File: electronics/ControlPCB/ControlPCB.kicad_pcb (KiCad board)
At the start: 2 copper layers, 119.6 x 90.4 mm, 44 parts, among them CON1 12VINPUT, P1 Opto1, P2 Opto2, P3 Opto3, P4 Opto4, P5 Opto5, P6 Opto6, P7 Tool, U1 POLOLU_A4988, U2 POLOLU_A4988, U3 POLOLU_A4988, U4 POLOLU_A4988, U5 POLOLU_A4988, U6 POLOLU_A4988, U7 POLOLU_A4988

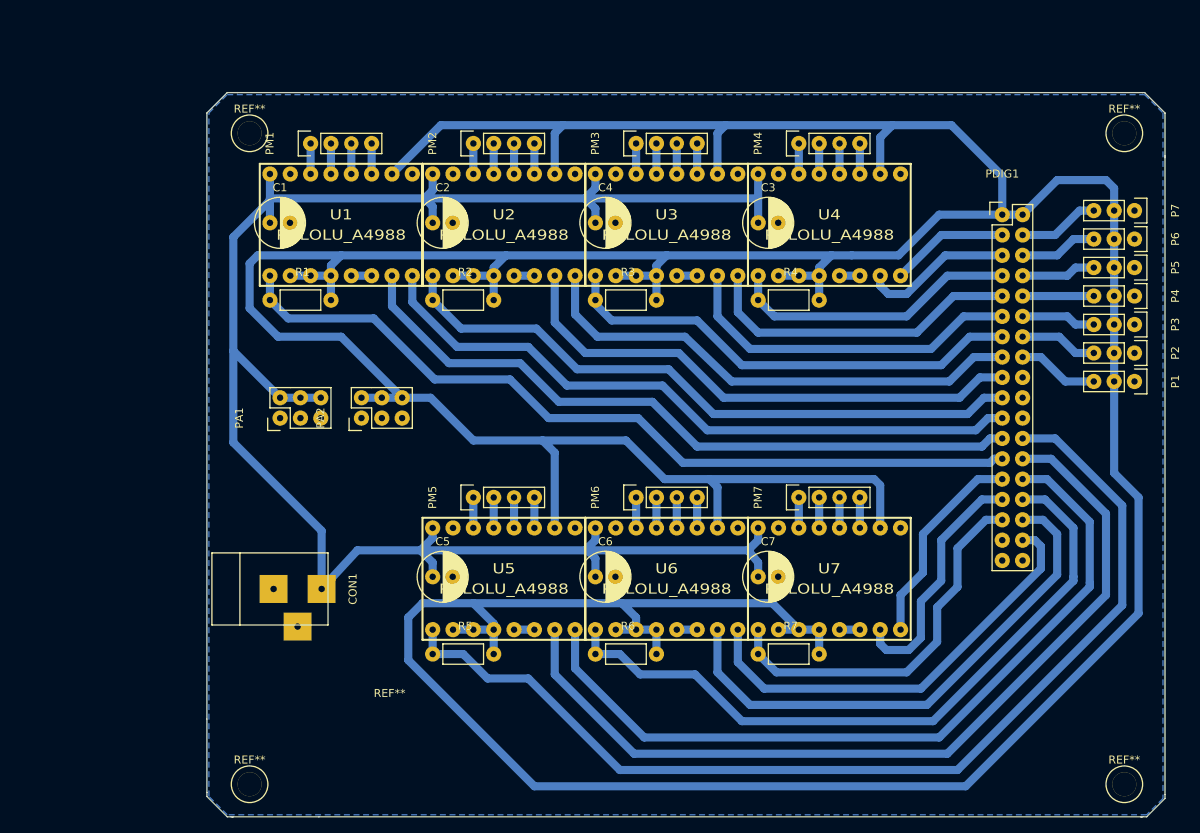
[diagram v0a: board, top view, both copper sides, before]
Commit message: PCB update
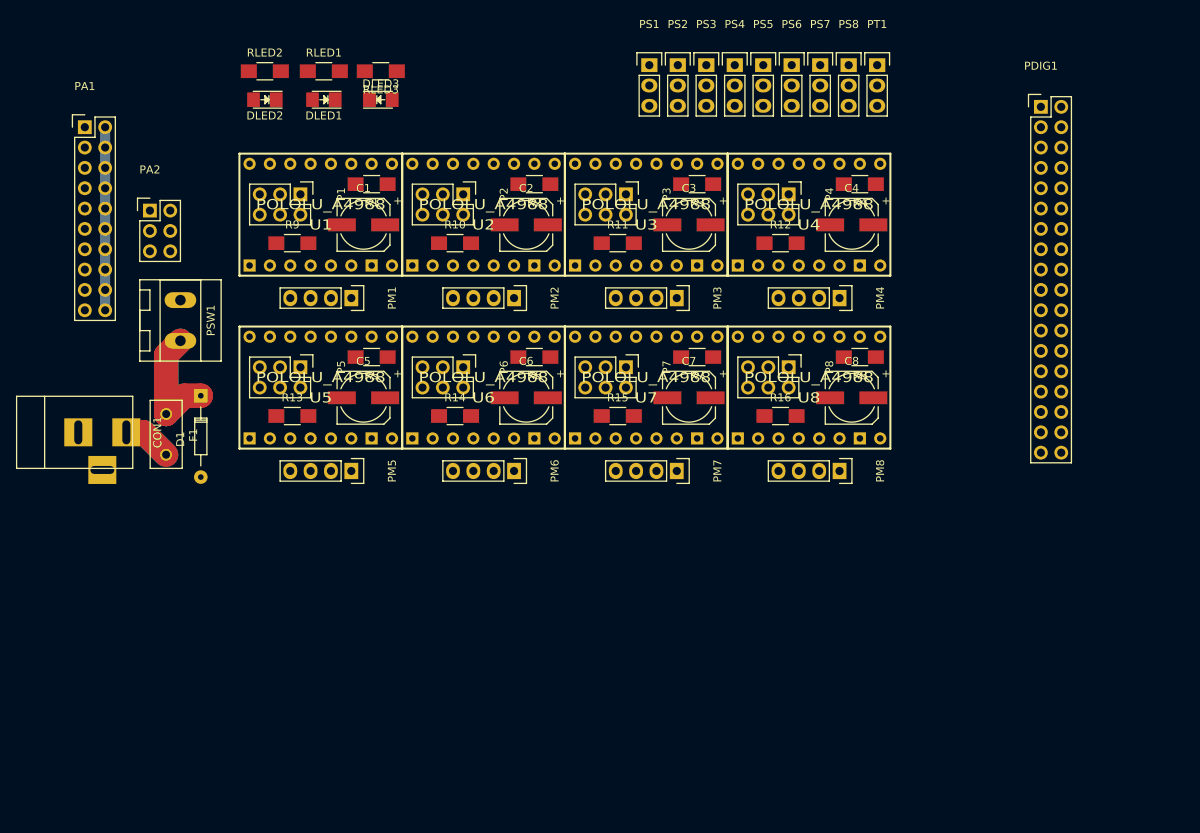
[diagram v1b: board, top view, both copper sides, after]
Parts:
- removed REF**: Symbol_OSHW-Logo_CopperTop_BIG, Symbols:Symbol_OSHW-Logo_CopperTop_BIG
- removed REF** (x4): 1pin, Connect:1pin
- added C8: CP1_Small, Capacitors_SMD:c_elec_6.3x5.7, F.Cu at (166.6, 91.4)
- added D1: D_Small, Diodes_ThroughHole:Diode_DO-35_SOD27_Horizontal_RM10, F.Cu at (85.3, 91.2)
- added DLED1: LEDFAN, LEDs:LED_1206, F.Cu at (100.7, 54.2)
- added DLED2: LED12V, LEDs:LED_1206, F.Cu at (93.3, 54.2)
- added DLED3: LED5V, LEDs:LED_1206, F.Cu at (107.8, 54.2)
- added F1: F_Small, Fuse_Holders_and_Fuses:Fuse_TE5_Littlefuse-395Series, F.Cu at (81.0, 96.0)
- added P8: CONN_02X03, Pin_Headers:Pin_Header_Straight_2x03, F.Cu at (158.8, 87.6)
- added PM8: CONN_01X04, Pin_Headers:Pin_Header_Straight_1x04, F.Cu at (165.1, 100.6)
- added PS1: Opto1, Pin_Headers:Pin_Header_Straight_1x03, F.Cu at (141.4, 49.9)
- added PS2: Opto2, Pin_Headers:Pin_Header_Straight_1x03, F.Cu at (144.9, 49.9)
- added PS3: Opto3, Pin_Headers:Pin_Header_Straight_1x03, F.Cu at (148.5, 49.9)
- added PS4: Opto4, Pin_Headers:Pin_Header_Straight_1x03, F.Cu at (152.0, 49.9)
- added PS5: Opto5, Pin_Headers:Pin_Header_Straight_1x03, F.Cu at (155.6, 49.9)
- added PS6: Opto6, Pin_Headers:Pin_Header_Straight_1x03, F.Cu at (159.1, 49.9)
- added PS7: Opto7, Pin_Headers:Pin_Header_Straight_1x03, F.Cu at (162.7, 49.9)
- added PS8: Opto8, Pin_Headers:Pin_Header_Straight_1x03, F.Cu at (166.2, 49.9)
- added PSW1: CONN_01X02, Connect:AK300-2, F.Cu at (82.8, 84.3)
- added PT1: Tool, Pin_Headers:Pin_Header_Straight_1x03, F.Cu at (169.8, 49.9)
- added R10: R, Resistors_SMD:R_1206_HandSoldering, F.Cu at (117.1, 72.1)
- added R11: R, Resistors_SMD:R_1206_HandSoldering, F.Cu at (137.4, 72.1)
- added R12: R, Resistors_SMD:R_1206_HandSoldering, F.Cu at (157.7, 72.1)
- added R13: R, Resistors_SMD:R_1206_HandSoldering, F.Cu at (96.8, 93.7)
- added R14: R, Resistors_SMD:R_1206_HandSoldering, F.Cu at (117.1, 93.7)
- added R15: R, Resistors_SMD:R_1206_HandSoldering, F.Cu at (137.4, 93.7)
- added R16: R, Resistors_SMD:R_1206_HandSoldering, F.Cu at (157.7, 93.7)
- added R8: R, Resistors_SMD:R_1206_HandSoldering, F.Cu at (167.6, 86.4)
- added R9: R, Resistors_SMD:R_1206_HandSoldering, F.Cu at (96.8, 72.1)
- added RLED1: 560, Resistors_SMD:R_1206_HandSoldering, F.Cu at (100.7, 50.7)
- added RLED2: 560, Resistors_SMD:R_1206_HandSoldering, F.Cu at (93.3, 50.7)
- added RLED3: 220, Resistors_SMD:R_1206_HandSoldering, F.Cu at (107.8, 50.7)
- added U8: POLOLU_A4988, Pololu:SWDIP8_.6W, F.Cu at (161.3, 90.2)
- C1, C2, C3, C4, C5, C6, C7: footprint POL:C_Radial_D6.3_L11.2_P2.5THOR -> Capacitors_SMD:c_elec_6.3x5.7
- P1: value Opto1 -> CONN_02X03; footprint Pin_Header_Straight_1x03 -> Pin_Headers:Pin_Header_Straight_2x03
- P2: value Opto2 -> CONN_02X03; footprint POL:Pin_Header_Straight_1x03 -> Pin_Headers:Pin_Header_Straight_2x03
- P3: value Opto3 -> CONN_02X03; footprint POL:Pin_Header_Straight_1x03 -> Pin_Headers:Pin_Header_Straight_2x03
- P4: value Opto4 -> CONN_02X03; footprint POL:Pin_Header_Straight_1x03 -> Pin_Headers:Pin_Header_Straight_2x03
- P5: value Opto5 -> CONN_02X03; footprint POL:Pin_Header_Straight_1x03 -> Pin_Headers:Pin_Header_Straight_2x03
- P6: value Opto6 -> CONN_02X03; footprint POL:Pin_Header_Straight_1x03 -> Pin_Headers:Pin_Header_Straight_2x03
- P7: value Tool -> CONN_02X03; footprint POL:Pin_Header_Straight_1x03 -> Pin_Headers:Pin_Header_Straight_2x03
- PA1: footprint POL:Pin_Header_Straight_2x03 -> Pin_Headers:Pin_Header_Straight_2x10
- PA2: footprint POL:Pin_Header_Straight_2x03 -> Pin_Headers:Pin_Header_Straight_2x03
- PDIG1: footprint POL:Pin_Header_Straight_2x18 -> Pin_Headers:Pin_Header_Straight_2x18
- PM1, PM2, PM3, PM4, PM5, PM6, PM7: footprint POL:Pin_Header_Straight_1x04 -> Pin_Headers:Pin_Header_Straight_1x04
- R1, R2, R3, R4, R5, R6, R7: footprint POL:Resistor_Horizontal_RM7mm -> Resistors_SMD:R_1206_HandSoldering
- U1, U2, U3, U4, U5, U6, U7: footprint POL:POLA4988 -> Pololu:SWDIP8_.6W
- moved P1 106.7 mm to (97.8, 66.0)
- moved P5 104.9 mm to (97.8, 87.6)
- moved P2 86.1 mm to (118.1, 66.0)
- moved P6 85.3 mm to (118.1, 87.6)
- moved P7 66.4 mm to (138.4, 87.6)
- moved P3 65.5 mm to (138.4, 66.0)
- moved P4 45.0 mm to (158.8, 66.0)
- moved PA1 43.7 mm to (70.9, 57.7), turned to 0 degrees
- moved R6 37.9 mm to (127.0, 86.4), turned to 180 degrees
- moved R7 37.9 mm to (147.3, 86.4), turned to 180 degrees
- moved R5 37.9 mm to (106.7, 86.4), turned to 180 degrees
- moved PA2 37.0 mm to (79.0, 68.1), turned to 0 degrees
- moved U7 33.1 mm to (141.0, 90.2), turned to 0 degrees
- moved U5 33.1 mm to (100.3, 90.2), turned to 0 degrees
- moved U6 33.1 mm to (120.7, 90.2), turned to 0 degrees
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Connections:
- CON1 pad 1: +12V -> Net-(CON1-Pad1)
- P1 pad 1: GND -> VCC
- P1 pad 2: VCC -> Net-(P1-Pad2)
- P1 pad 3: SOPTO1 -> VCC
- P2 pad 1: GND -> VCC
- P2 pad 2: VCC -> Net-(P2-Pad2)
- P2 pad 3: SOPTO2 -> VCC
- P3 pad 1: GND -> VCC
- P3 pad 2: VCC -> Net-(P3-Pad2)
- P3 pad 3: SOPTO3 -> VCC
- P4 pad 1: GND -> VCC
- P4 pad 2: VCC -> Net-(P4-Pad2)
- P4 pad 3: SOPTO4 -> VCC
- P5 pad 1: GND -> VCC
- P5 pad 2: VCC -> Net-(P5-Pad2)
- P5 pad 3: SOPTO5 -> VCC
- P6 pad 1: GND -> VCC
- P6 pad 2: VCC -> Net-(P6-Pad2)
- P6 pad 3: SOPTO6 -> VCC
- P7 pad 1: GND -> VCC
- P7 pad 2: VCC -> Net-(P7-Pad2)
- P7 pad 3: STOOL -> VCC
- PA1 pad 2: +12V -> VDD
- PA1 pad 4: +12V -> VDD
- PA1 pad 6: +12V -> VDD
- PDIG1 pad 10: SOPTO4 -> STEPM8
- PDIG1 pad 11: STEPM3 -> DIRM1
- PDIG1 pad 12: SOPTO3 -> DIRM2
- PDIG1 pad 13: ENABLEM3 -> DIRM3
- PDIG1 pad 14: SOPTO2 -> DIRM4
- PDIG1 pad 15: DIRM2 -> DIRM5
- PDIG1 pad 16: SOPTO1 -> DIRM6
- PDIG1 pad 17: STEPM2 -> DIRM7
- PDIG1 pad 18: Net-(PDIG1-Pad18) -> DIRM8
- PDIG1 pad 19: ENABLEM2 -> Net-(PDIG1-Pad19)
- PDIG1 pad 21: DIRM1 -> ENABLEM
- PDIG1 pad 22: Net-(PDIG1-Pad22) -> STOOL
- PDIG1 pad 23: STEPM1 -> SOPTO1
- PDIG1 pad 24: ENABLEM5 -> SOPTO2
- PDIG1 pad 25: ENABLEM1 -> SOPTO3
- PDIG1 pad 26: STEPM5 -> SOPTO4
- PDIG1 pad 27: DIRM7 -> SOPTO5
- PDIG1 pad 28: DIRM5 -> SOPTO6
- PDIG1 pad 29: STEPM7 -> SOPTO7
- PDIG1 pad 3: DIRM4 -> STEPM1
- PDIG1 pad 30: ENABLEM6 -> SOPTO8
- PDIG1 pad 31: ENABLEM7 -> Net-(PDIG1-Pad31)
- PDIG1 pad 32: STEPM6 -> Net-(PDIG1-Pad32)
- PDIG1 pad 34: DIRM6 -> Net-(PDIG1-Pad34)
- PDIG1 pad 4: STOOL -> STEPM2
- PDIG1 pad 5: STEPM4 -> STEPM3
- PDIG1 pad 6: SOPTO6 -> STEPM4
- PDIG1 pad 7: ENABLEM4 -> STEPM5
- PDIG1 pad 8: SOPTO5 -> STEPM6
- PDIG1 pad 9: DIRM3 -> STEPM7
- R1 pad 1: ENABLEM1 -> ENABLEM
- R2 pad 1: ENABLEM2 -> ENABLEM
- R3 pad 1: ENABLEM3 -> ENABLEM
- R4 pad 1: ENABLEM4 -> ENABLEM
- R5 pad 1: ENABLEM5 -> ENABLEM
- R6 pad 1: ENABLEM6 -> ENABLEM
- R7 pad 1: ENABLEM7 -> ENABLEM
- U1 pad 10: VCC -> Net-(P1-Pad2)
- U1 pad 11: VCC -> Net-(P1-Pad4)
- U1 pad 12: VCC -> Net-(P1-Pad6)
- U1 pad 9: ENABLEM1 -> ENABLEM
- U2 pad 10: VCC -> Net-(P2-Pad2)
- U2 pad 11: VCC -> Net-(P2-Pad4)
- U2 pad 12: VCC -> Net-(P2-Pad6)
- U2 pad 9: ENABLEM2 -> ENABLEM
- U3 pad 10: VCC -> Net-(P3-Pad2)
- U3 pad 11: VCC -> Net-(P3-Pad4)
- U3 pad 12: VCC -> Net-(P3-Pad6)
- U3 pad 9: ENABLEM3 -> ENABLEM
- U4 pad 10: VCC -> Net-(P4-Pad2)
- U4 pad 11: VCC -> Net-(P4-Pad4)
- U4 pad 12: VCC -> Net-(P4-Pad6)
- U4 pad 9: ENABLEM4 -> ENABLEM
- U5 pad 10: VCC -> Net-(P5-Pad2)
- U5 pad 11: VCC -> Net-(P5-Pad4)
- U5 pad 12: VCC -> Net-(P5-Pad6)
- U5 pad 9: ENABLEM5 -> ENABLEM
- U6 pad 10: VCC -> Net-(P6-Pad2)
- U6 pad 11: VCC -> Net-(P6-Pad4)
- U6 pad 12: VCC -> Net-(P6-Pad6)
- U6 pad 9: ENABLEM6 -> ENABLEM
- U7 pad 10: VCC -> Net-(P7-Pad2)
- U7 pad 11: VCC -> Net-(P7-Pad4)
- U7 pad 12: VCC -> Net-(P7-Pad6)
- U7 pad 9: ENABLEM7 -> ENABLEM
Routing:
- net VCC: track 635.6 -> 0.00 mm
- net +12V: track 232.8 -> 0.00 mm
- net ENABLEM5: track 132.0 -> 0.00 mm
- net STEPM5: track 110.1 -> 0.00 mm
- net ENABLEM1: track 103.1 -> 0.00 mm
- net DIRM5: track 99.2 -> 0.00 mm
- net ENABLEM6: track 87.9 -> 0.00 mm
- net STEPM1: track 87.7 -> 0.00 mm
- net DIRM1: track 84.2 -> 0.00 mm
- net ENABLEM2: track 80.9 -> 0.00 mm
- net STEPM2: track 66.7 -> 0.00 mm
- net STEPM6: track 66.3 -> 0.00 mm
- net DIRM2: track 62.8 -> 0.00 mm
- net ENABLEM3: track 59.0 -> 0.00 mm
- net DIRM6: track 54.9 -> 0.00 mm
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- removed copper zone on B.Cu, net GND
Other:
- board outline removed
- net class Default: clearance 0.2 -> 0; trace_width 1.016 -> 0.254; via_dia 0.6 -> 0.6096; via_drill 0.4 -> 0.3048
- rule pad_to_mask_clearance: 0.2 -> 0
- rule trace_clearance: 0.2 -> 0
- rule trace_min: 0.2 -> 0.1524
- rule via_min_drill: 0.3 -> 0.3048
- rule via_min_size: 0.4 -> 0.6096
